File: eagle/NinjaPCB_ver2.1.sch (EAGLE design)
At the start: 70 parts, among them IC1 ANALOGSW_AD_SOT23-6, IC2 NAU7802, Q1 IRLB3813PBF, Q2 CJ2302, Q3 CJ2302, Q4 S9013, Q5 S9013, Q6 S9013

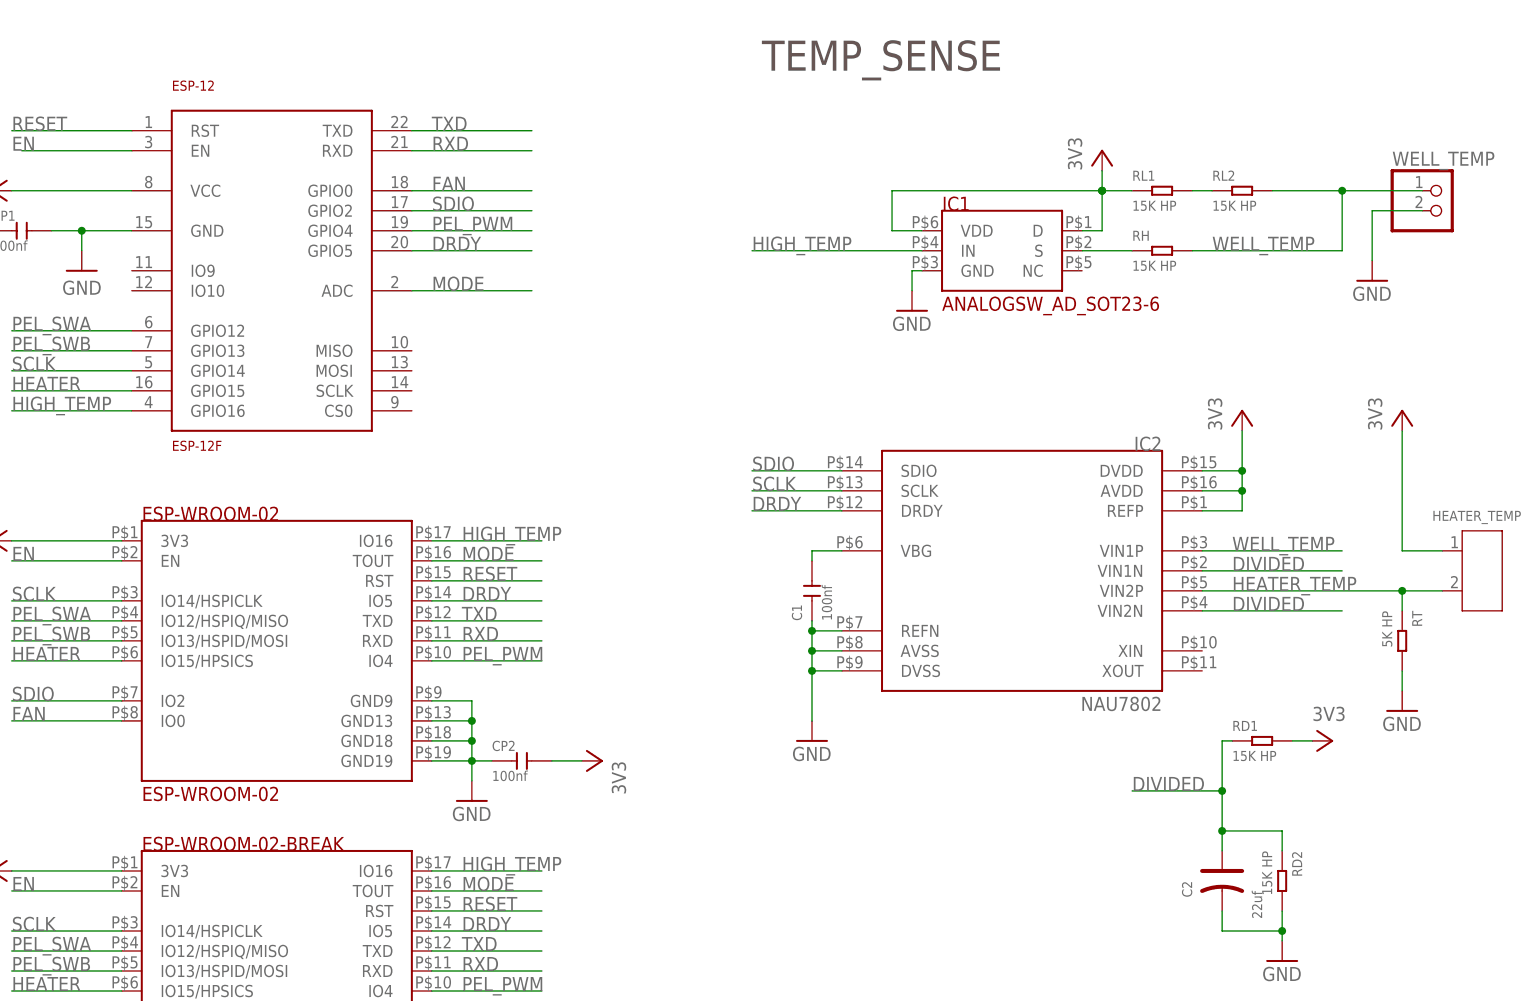
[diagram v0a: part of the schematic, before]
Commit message: minor update of silk
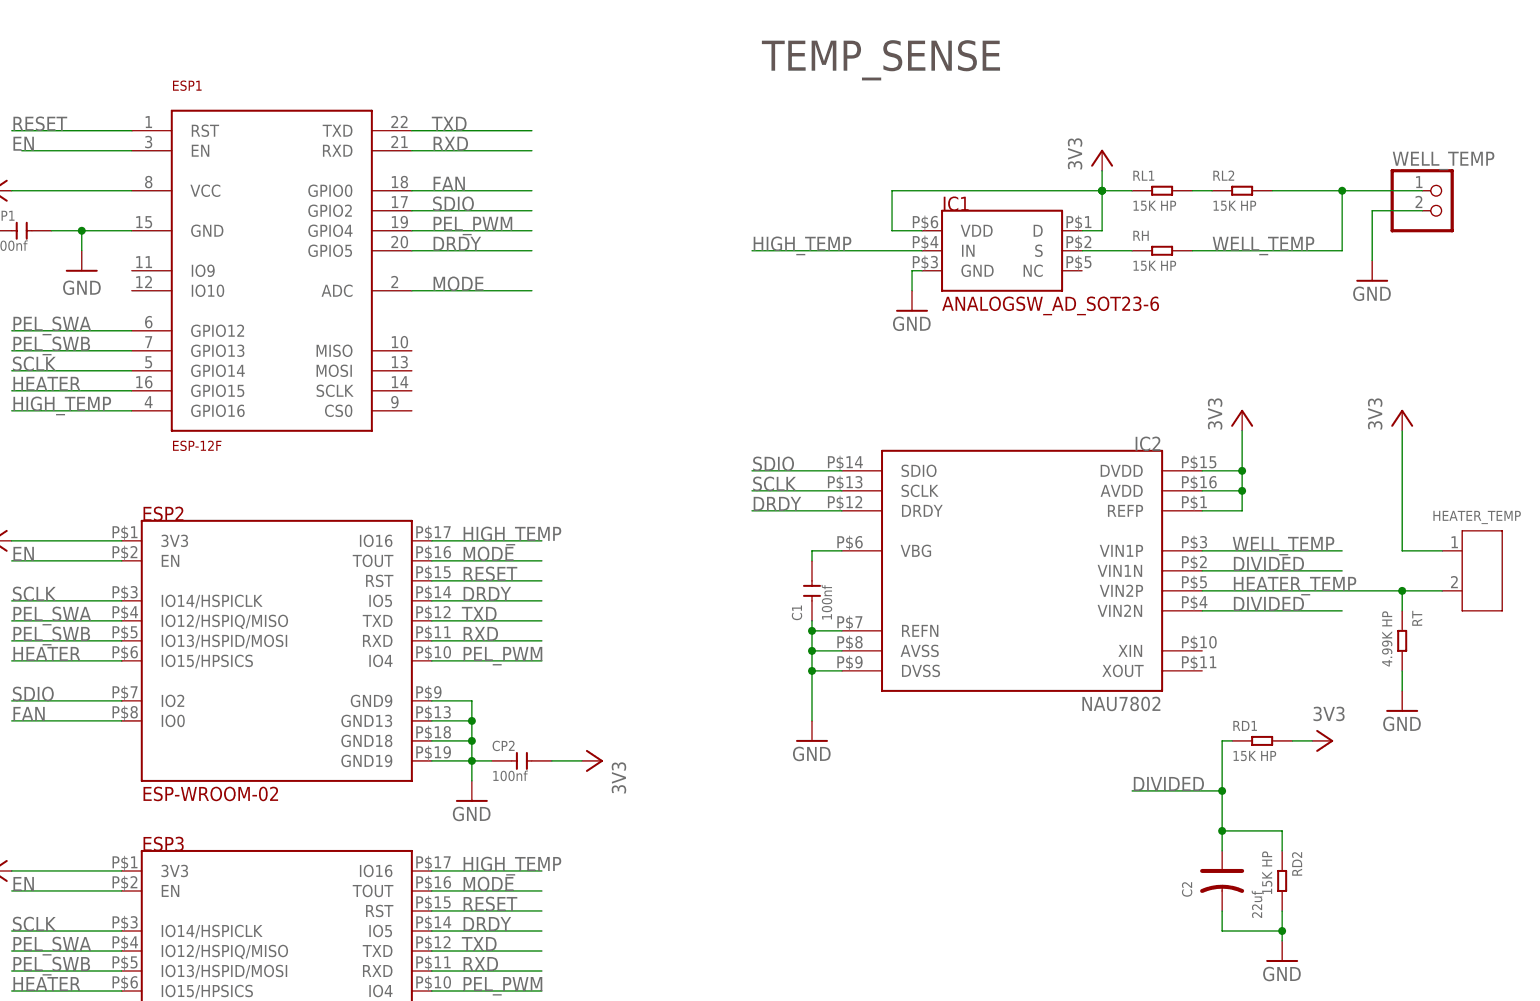
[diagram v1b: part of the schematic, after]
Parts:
- RT: value 5K HP -> 4.99K HP
- renumbered ESP-12 to ESP1, ESP-WROOM-02 to ESP2, ESP-WROOM-02-BREAK to ESP3
